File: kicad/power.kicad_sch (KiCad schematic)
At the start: 27 parts, among them J2 Conn_01x04_Socket, J3 Eurorack Power Small, J6 Conn_01x04_Header, U1 TL074, U2 CD4093, U3 TL072, U4 LM13700, U5 TL074, U6 LM13700, U7 LM13700

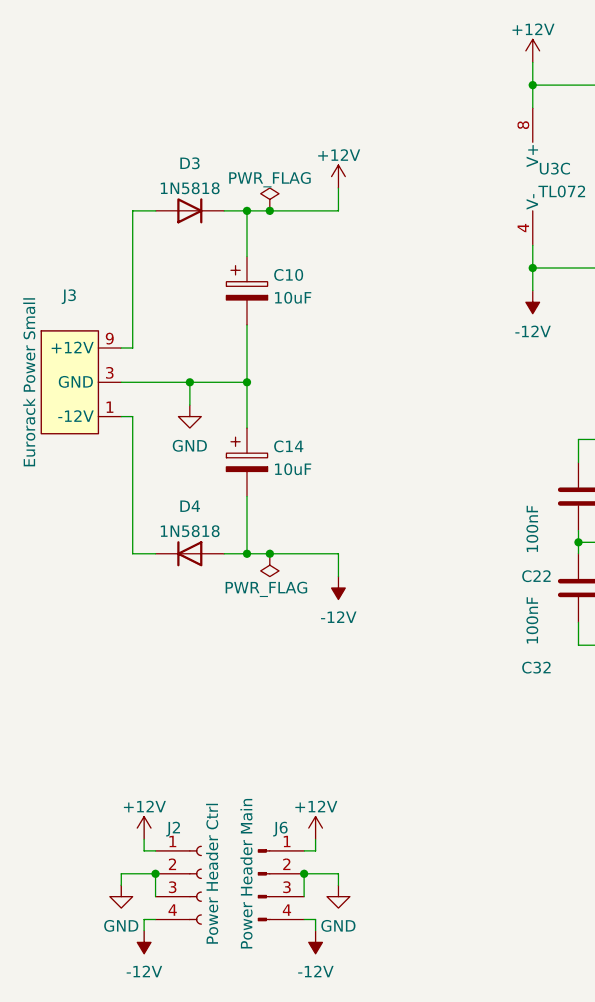
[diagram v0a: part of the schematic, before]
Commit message: Update kicad project for v7
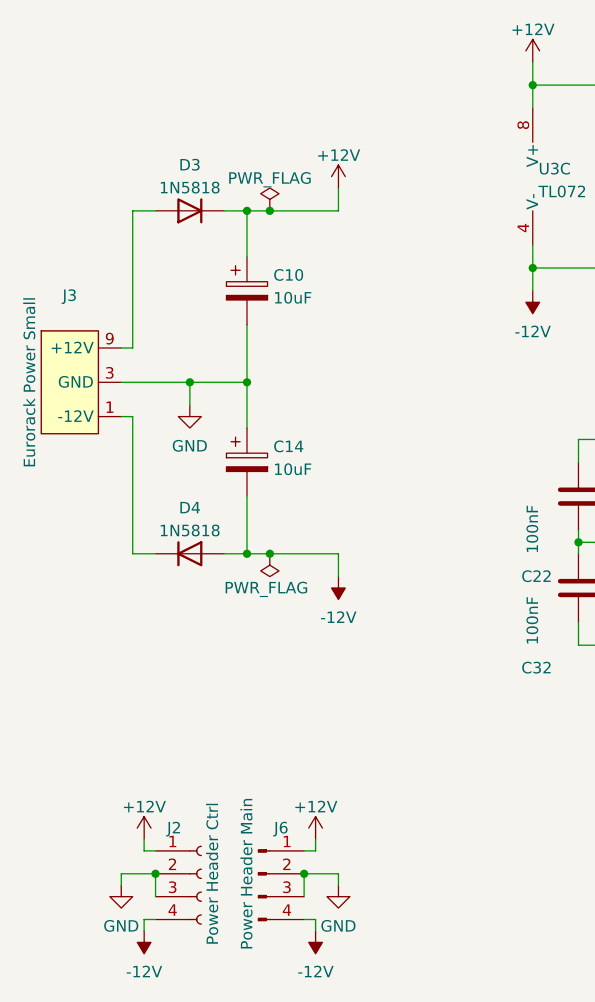
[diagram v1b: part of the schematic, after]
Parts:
- C10, C14: footprint rumblesan-standard-parts:CP_Radial_D5.0mm_P2.00mm -> Rumblesan_Standard_Parts:CP_Radial_D5.0mm_P2.00mm
- C13, C22, C25, C26, C28, C31, C32, C34, C35, C4, C5, C8, C9: footprint rumblesan-standard-parts:C_Rect_L7.0mm_W3.5mm_P5.00mm -> Rumblesan_Standard_Parts:C_Rect_L7.0mm_W3.5mm_P5.00mm
- D3, D4: footprint rumblesan-standard-parts:D_DO-41_SOD81_P10.16mm_Horizontal -> Rumblesan_Standard_Parts:D_DO-41_SOD81_P10.16mm_Horizontal
- J2: symbol Connector:Conn_01x04_Female -> Connector:Conn_01x04_Socket
- J3: footprint eurorack-power:Eurorack_PowerHeader_2x05_P2.54mm_Shrouded -> Eurorack_Power:Eurorack_PowerHeader_2x05_P2.54mm_Shrouded; symbol Eurorack_Hardware:Eurorack Power Small -> Eurorack_Power:Eurorack Power Small
- J6: symbol Connector:Conn_01x04_Male -> Connector:Conn_01x04_Pin
- U1, U2, U5: footprint rumblesan-standard-parts:DIP-14_W7.62mm_Socket -> Rumblesan_Standard_Parts:DIP-14_W7.62mm_Socket
- U3: footprint rumblesan-standard-parts:DIP-8_W7.62mm_Socket -> Rumblesan_Standard_Parts:DIP-8_W7.62mm_Socket
- U4, U6, U7: footprint rumblesan-standard-parts:DIP-16_W7.62mm_Socket -> Rumblesan_Standard_Parts:DIP-16_W7.62mm_Socket
